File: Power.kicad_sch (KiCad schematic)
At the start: 46 parts, among them J21 Conn_01x06, Q2 MBT2222ADW1T1, Q3 MBT2222ADW1T1, U6 TPS7A4501DCQT, U7 TPS54226PWPR, U8 BQ25883RGER, U9 ADM1176-1ARMZ-R7

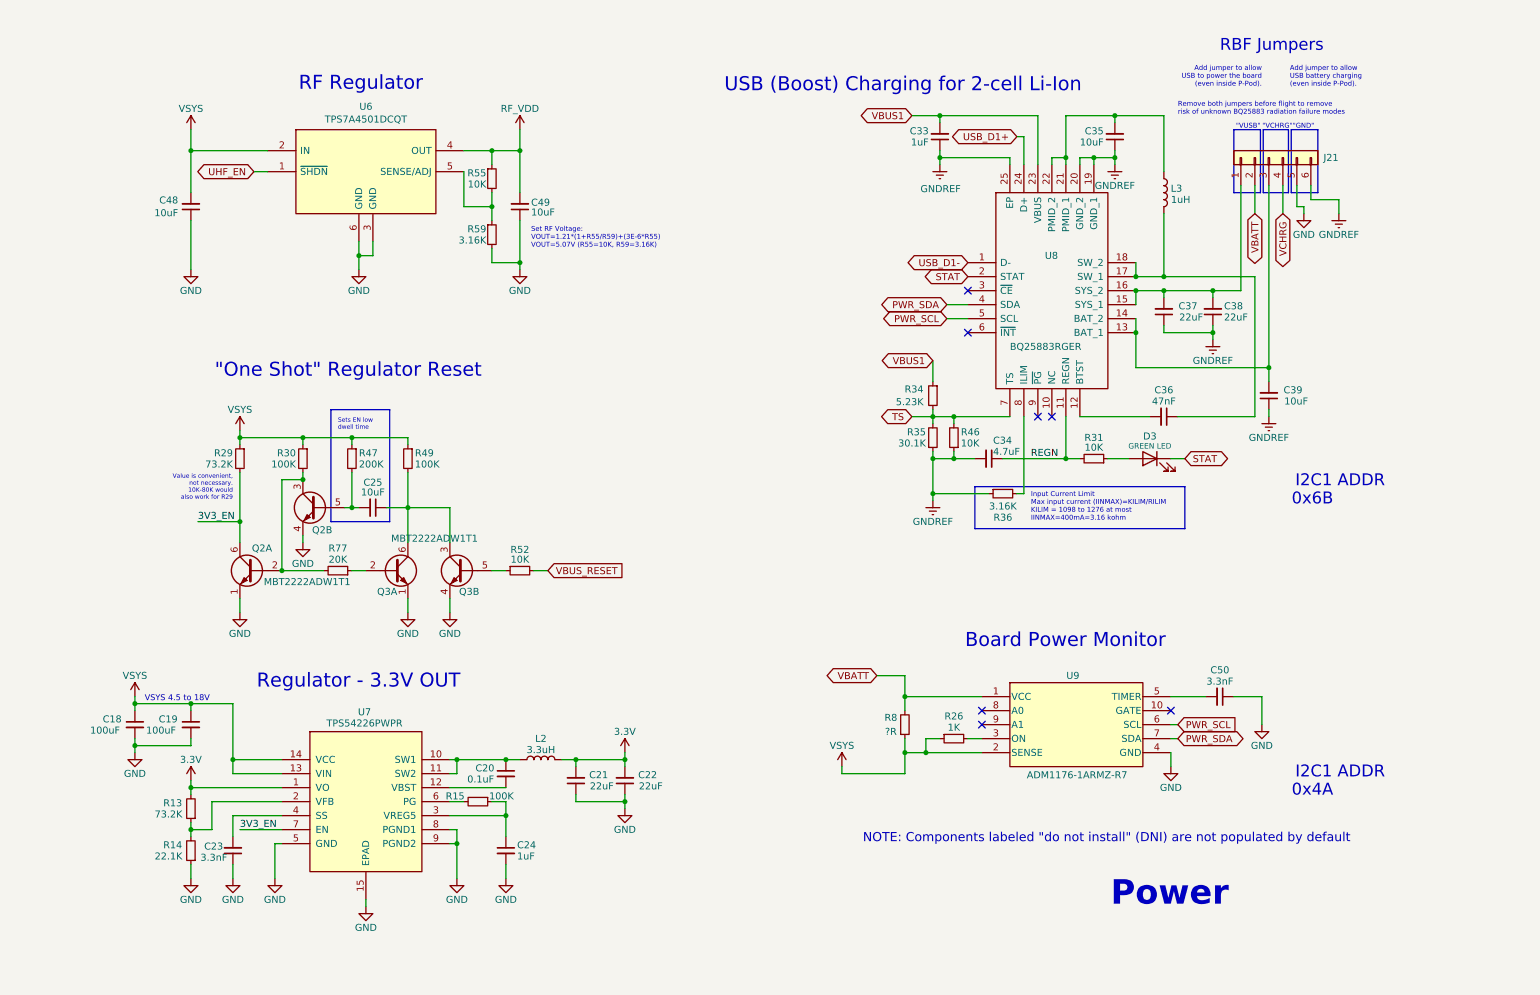
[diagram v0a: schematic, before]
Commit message: v1.1 Schematic
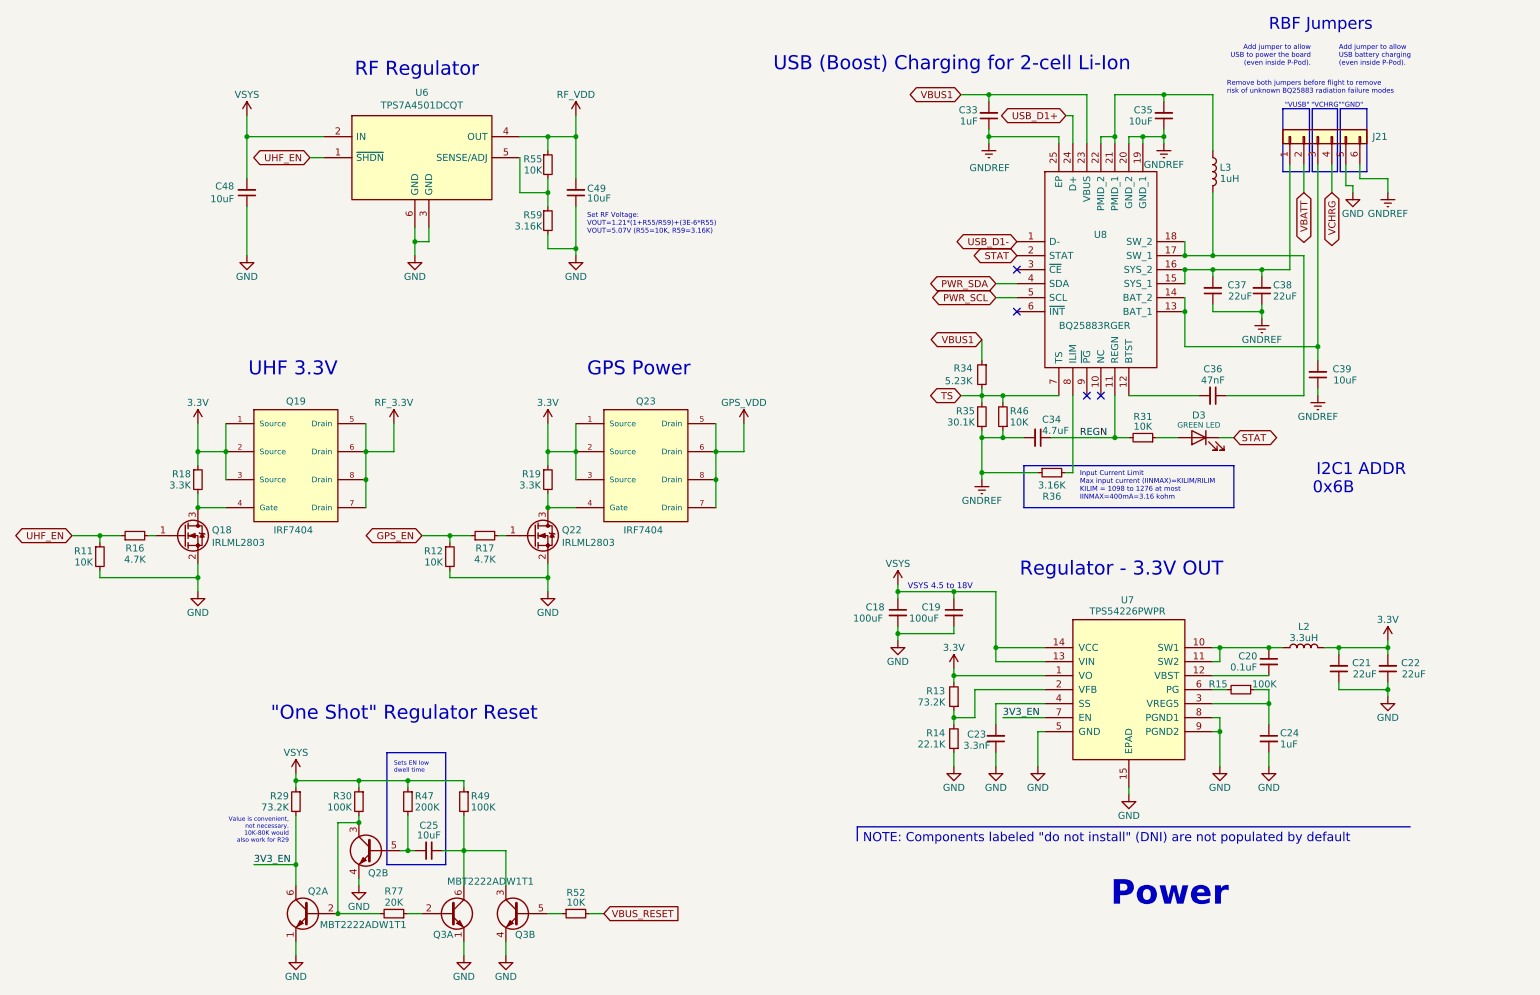
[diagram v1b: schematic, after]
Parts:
- removed C50: 3.3nF, Capacitor_SMD:C_0603_1608Metric, symbol Device:C_Small
- removed R26: 1K, Resistor_SMD:R_0603_1608Metric, symbol Device:R_Small
- removed R8: ?R, Resistor_SMD:R_2512_6332Metric, symbol Device:R_Small
- removed U9: ADM1176-1ARMZ-R7, Package_SO:MSOP-10_3x3mm_P0.5mm, symbol Mainboard:ADM1176-1ARMZ-R7
- added Q18, Q22: IRLML2803, Package_TO_SOT_SMD:SOT-23, symbol Mainboard:IRLML2803
- added Q19, Q23: IRF7404, Package_SO:SOIC-8_3.9x4.9mm_P1.27mm, symbol Mainboard:IRF7404
- added R11, R12: 10K, Resistor_SMD:R_0603_1608Metric, symbol Device:R_Small
- added R16, R17: 4.7K, Resistor_SMD:R_0603_1608Metric, symbol Device:R_Small
- added R18, R19: 3.3K, Resistor_SMD:R_0603_1608Metric, symbol Device:R_Small
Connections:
- net 3.3V: now also Q19.1 (Source), Q19.2 (Source), Q19.3 (Source), Q23.1 (Source), Q23.2 (Source), Q23.3 (Source), R18.1, R19.1
- net GND: now also Q18.2 (S), Q22.2 (S), R11.2, R12.2
- net UHF_EN: now also R11.1, R16.1
- new net: Q18.1 (G), R16.2
- new net: Q18.3 (D), Q19.4 (Gate), R18.2
- new net: Q22.1 (G), R17.2
- new net: Q22.3 (D), Q23.4 (Gate), R19.2
- new net GPS_EN: R12.1, R17.1
- new net GPS_VDD: Q23.5 (Drain), Q23.6 (Drain), Q23.7 (Drain), Q23.8 (Drain)
- new net RF_3.3V: Q19.5 (Drain), Q19.6 (Drain), Q19.7 (Drain), Q19.8 (Drain)
- no-connect marks 7 -> 4
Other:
- note added: "GPS Power"
- note added: "UHF 3.3V"
- note removed: "0x4A"
- note removed: "Board Power Monitor"
- moved on the sheet: C18, C19, C20, C21, C22, C23, C24, C25, C33, C34, C35, C36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
